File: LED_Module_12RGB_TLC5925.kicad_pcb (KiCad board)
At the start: 2 copper layers, 120.4 x 46.4 mm, 28 parts, among them J1 Conn_01x02_Pin, J2 Conn_02x05_Counter_Clockwise, J3 Conn_02x05_Counter_Clockwise, U1 TLC5925IPWR, U3 AMS1117-3.3

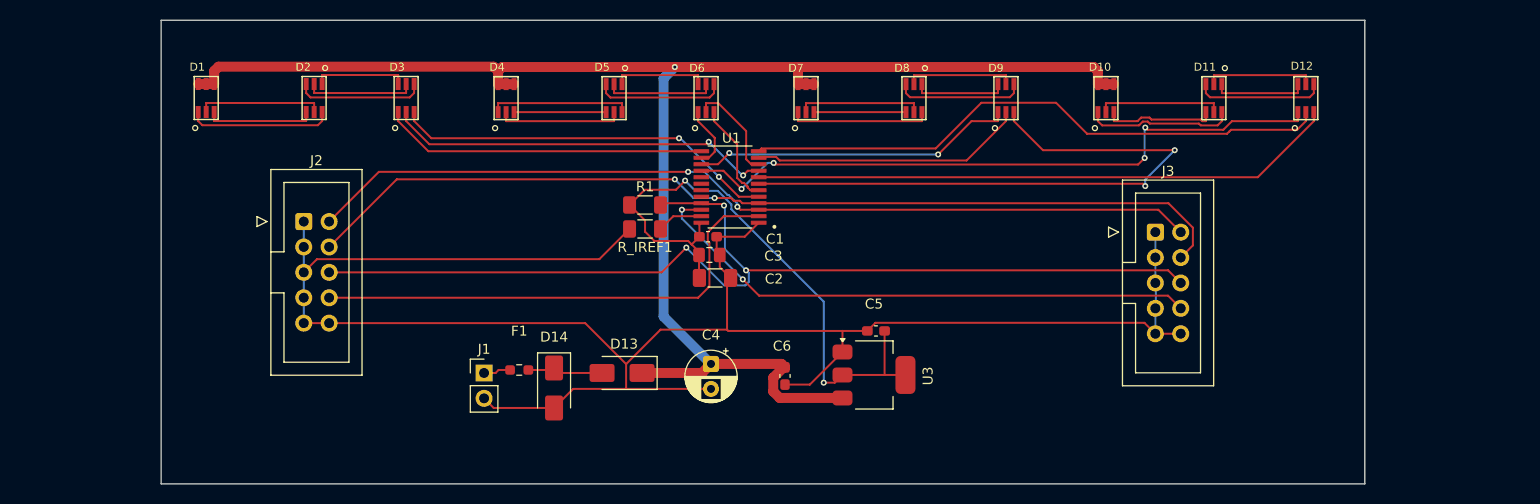
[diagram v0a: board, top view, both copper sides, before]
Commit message: v1 ok
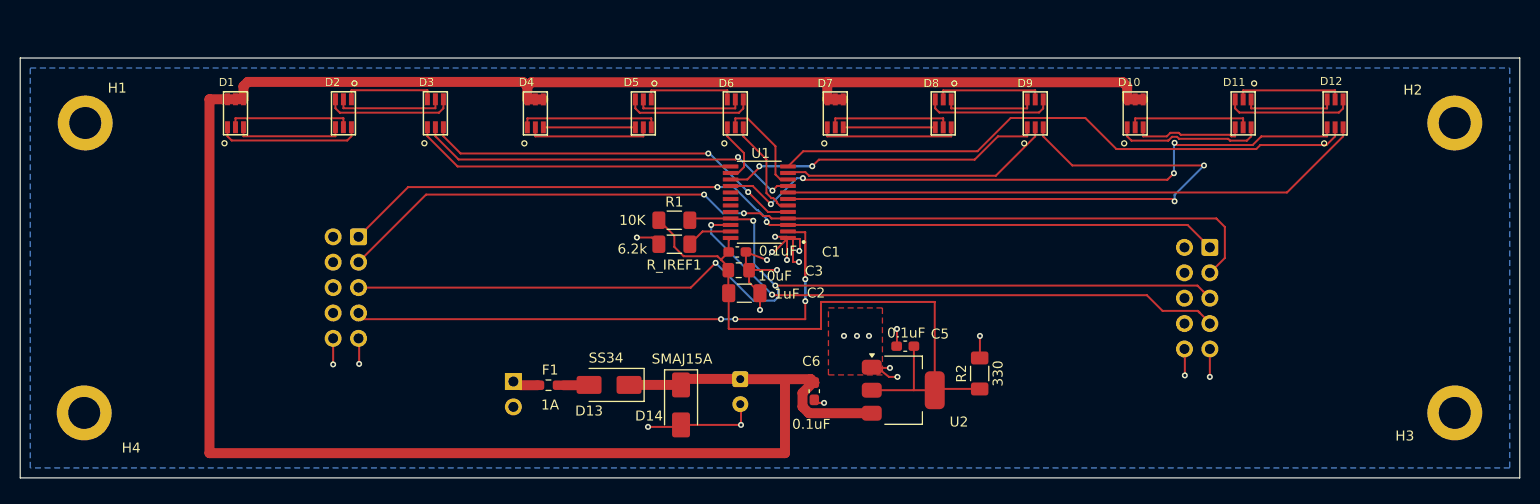
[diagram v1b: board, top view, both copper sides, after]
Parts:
- added H1: 3.2mm_M3, footprints:MountingHole_3.2mm_M3, F.Cu at (66.5, 78.5)
- added H2: 3.2mm_M3, footprints:MountingHole_3.2mm_M3, F.Cu at (203.5, 78.5)
- added H3: 3.2mm_M3, footprints:MountingHole_3.2mm_M3, F.Cu at (203.5, 107.5)
- added H4: 3.2mm_M3, footprints:MountingHole_3.2mm_M3, F.Cu at (66.4, 107.5)
- added R2: 330, Resistor_SMD:R_1206_3216Metric_Pad1.30x1.75mm_HandSolder, F.Cu at (156.0, 103.6)
- C4, J1, J2, J3: moved to B.Cu
- moved D14 12.8 mm to (126.1, 106.7)
- moved J2 5.69 mm to (93.8, 89.9), turned to 180 degrees
- moved J3 5.66 mm to (179.0, 90.9), turned to 180 degrees
- moved C2 3.30 mm to (132.4, 95.5)
- moved C4 3.30 mm to (132.0, 104.1)
- moved C5 3.30 mm to (148.5, 100.8)
- moved C6 3.30 mm to (139.4, 105.3)
- moved D1 3.30 mm to (81.9, 77.5)
- moved D2 3.30 mm to (91.9, 77.5)
- moved D3 3.30 mm to (101.9, 77.5)
- moved R_IREF1 3.30 mm to (125.4, 90.6)
- moved C3 3.30 mm to (131.9, 93.2)
- moved D10 3.30 mm to (171.9, 77.5)
- moved D11 3.30 mm to (181.9, 77.5)
- moved D12 3.30 mm to (191.9, 77.5)
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- renumbered U3 to U2
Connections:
- D14 pad 1: Net-(D13-A) -> +12V
- J2 pad 1: GND -> CLK
- J2 pad 2: CLK -> GND
- J2 pad 3: GND -> LE
- J2 pad 4: LE -> GND
- J2 pad 5: GND -> OE
- J2 pad 6: OE -> GND
- J2 pad 7: GND -> SDI
- J2 pad 8: SDI -> GND
- J3 pad 1: GND -> CLK
- J3 pad 2: CLK -> GND
- J3 pad 3: GND -> LE
- J3 pad 4: LE -> GND
- J3 pad 5: GND -> OE
- J3 pad 6: OE -> GND
- J3 pad 7: GND -> SDO
- J3 pad 8: SDO -> GND
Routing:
- net GND: track 194.3 -> 10.9 mm, vias 0 -> 23
- net SDI: track 49.8 -> 5.98 mm, vias 0 -> 4
- net +12V: track 158.2 -> 118.8 mm, vias 1 -> 0
- net Net-(D13-A): track 7.66 -> 0.00 mm
- net /Connectors/12V IN: track 2.72 -> 0.00 mm
- net LE: track 94.7 -> 96.0 mm
- net CLK: track 89.9 -> 89.0 mm
- net VDD_3V3: track 61.6 -> 60.8 mm, vias 2 -> 0
- net OE: track 104.3 -> 104.8 mm
- added copper zone on B.Cu, net GND
- added copper zone on F.Cu, net GND
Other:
- board size 120.4 x 46.4 mm -> 150 x 42 mm
- board text added: "+12V"
- board text added: "CLK"
- board text added: "GND"
- board text added: "IN"
- board text added: "LE"
- board text added: "OE"
- board text added: "OUT"
- board text added: "POWER"
- board text added: "SDI"
- board text added: "SDO"
